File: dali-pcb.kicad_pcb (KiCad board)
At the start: 2 copper layers, 180.5 x 113 mm, 62 parts, among them J1 12-22.5V DC, J10 5V DC, J11 5V DC, J12 5V DC, J13 5V DC, J14 5V DC, J15 GND, J2 DALI BUS, J20 LOLIN-S3 (L), J21 LOLIN-S3 (R), J22 ESP32-S3-DEVKITC-1 (L), J23 ESP32-S3-DEVKITC-1 (R), J24 LOLIN-S3-MINI (L), J25 LOLIN-S3-MINI (R), J26 LOLIN-S2-MINI (L), J27 LOLIN-S2-MINI (R), J3 DALI BUS, J30 FTDI-MCU, J31 UART-DALI, J4 DALI BUS, J40 A10-0, J41 A5-0, J42 A5-5, J43 A2-0, J44 A2-2, J45 A2-4, J46 A2-6, J47 A2-8, J50 D8-11, J51 D4-11, J52 D4-16, J53 D2-11, J54 D2-13, J55 D2-16, J56 D2-18, J60 D1-11, J61 D1-12, J62 D1-13, J63 D1-14, Q1 PZT2222A, Q2 MMBT2222A, U1 TCLT1000, U2 TCLT1000

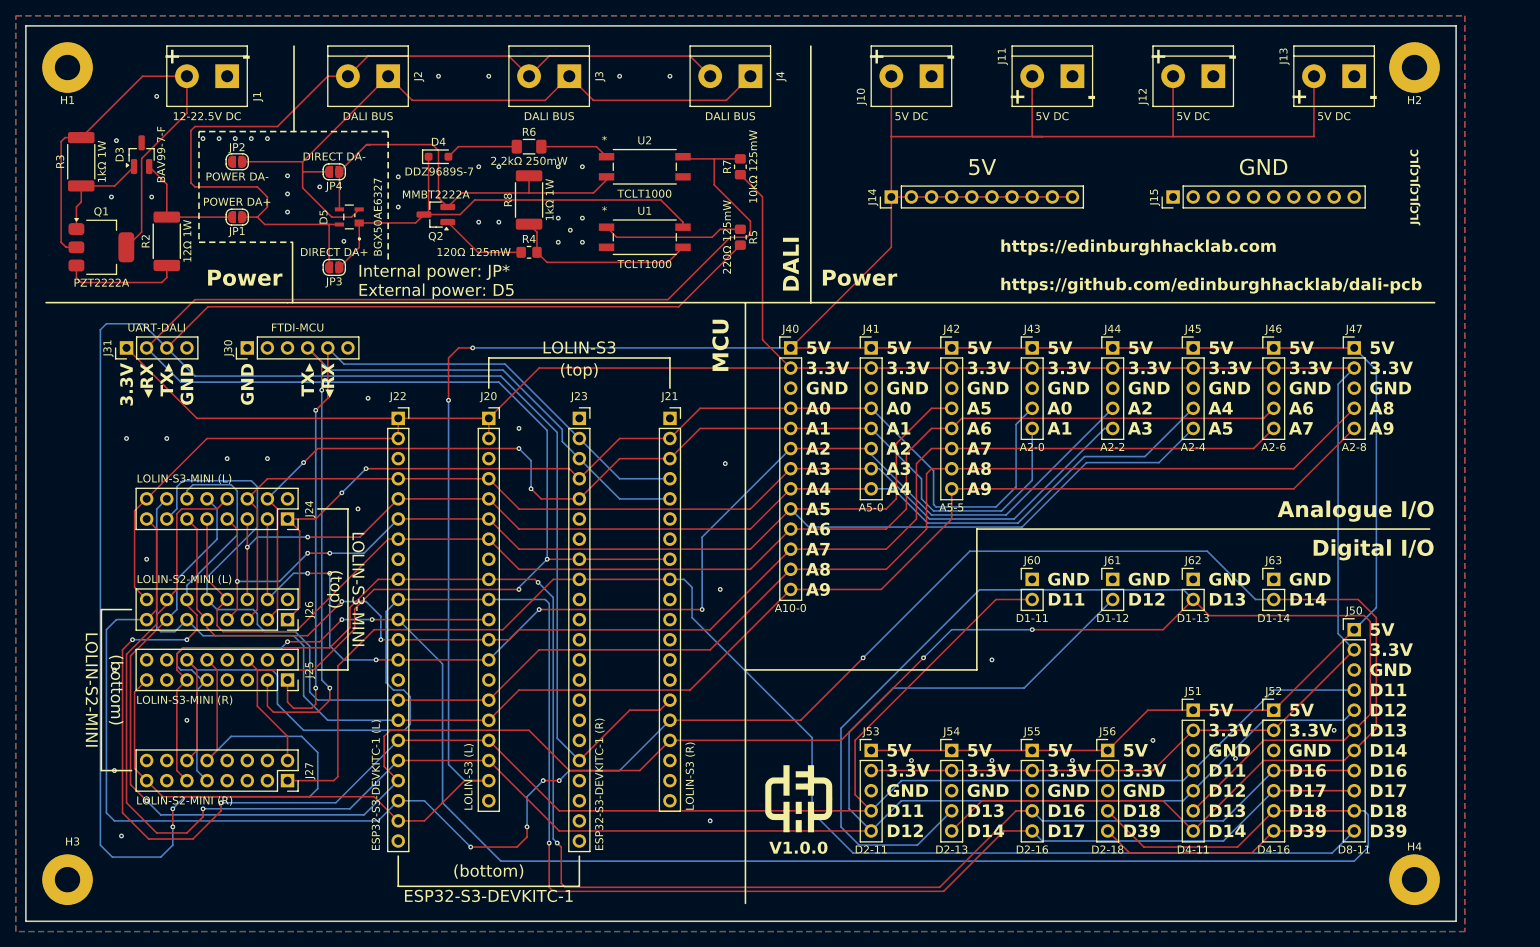
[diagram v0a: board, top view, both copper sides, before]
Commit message: Remove the kitchen sink
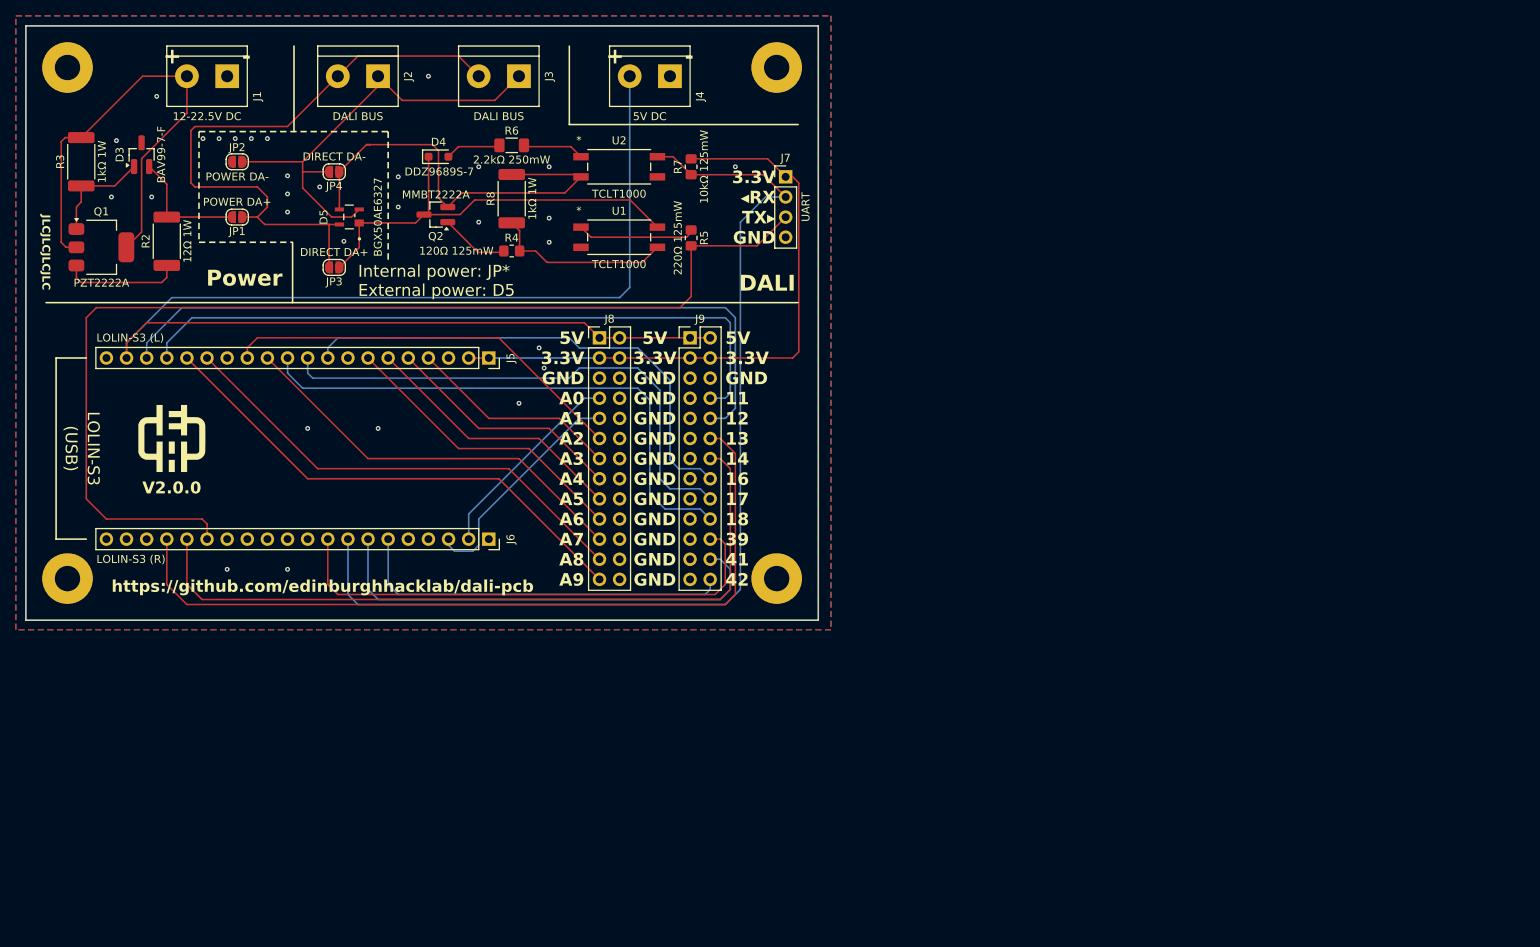
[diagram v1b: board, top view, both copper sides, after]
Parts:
- removed J11, J12, J13: 5V DC, TerminalBlock:TerminalBlock_bornier-2_P5.08mm
- removed J14: 5V DC, Connector_PinHeader_2.54mm:PinHeader_1x10_P2.54mm_Vertical
- removed J15: GND, Connector_PinHeader_2.54mm:PinHeader_1x10_P2.54mm_Vertical
- removed J22: ESP32-S3-DEVKITC-1 (L), Connector_PinSocket_2.54mm:PinSocket_1x22_P2.54mm_Vertical
- removed J23: ESP32-S3-DEVKITC-1 (R), Connector_PinSocket_2.54mm:PinSocket_1x22_P2.54mm_Vertical
- removed J24: LOLIN-S3-MINI (L), Connector_PinSocket_2.54mm:PinSocket_2x08_P2.54mm_Vertical
- removed J25: LOLIN-S3-MINI (R), Connector_PinSocket_2.54mm:PinSocket_2x08_P2.54mm_Vertical
- removed J26: LOLIN-S2-MINI (L), Connector_PinSocket_2.54mm:PinSocket_2x08_P2.54mm_Vertical
- removed J27: LOLIN-S2-MINI (R), Connector_PinSocket_2.54mm:PinSocket_2x08_P2.54mm_Vertical
- removed J30: FTDI-MCU, Connector_PinHeader_2.54mm:PinHeader_1x06_P2.54mm_Vertical
- removed the J4 at (106.7, 21.6)
- removed J41: A5-0, Connector_PinHeader_2.54mm:PinHeader_1x08_P2.54mm_Vertical
- removed J42: A5-5, Connector_PinHeader_2.54mm:PinHeader_1x08_P2.54mm_Vertical
- removed J43: A2-0, Connector_PinHeader_2.54mm:PinHeader_1x05_P2.54mm_Vertical
- removed J44: A2-2, Connector_PinHeader_2.54mm:PinHeader_1x05_P2.54mm_Vertical
- removed J45: A2-4, Connector_PinHeader_2.54mm:PinHeader_1x05_P2.54mm_Vertical
- removed J46: A2-6, Connector_PinHeader_2.54mm:PinHeader_1x05_P2.54mm_Vertical
- removed J47: A2-8, Connector_PinHeader_2.54mm:PinHeader_1x05_P2.54mm_Vertical
- removed J51: D4-11, Connector_PinHeader_2.54mm:PinHeader_1x07_P2.54mm_Vertical
- removed J52: D4-16, Connector_PinHeader_2.54mm:PinHeader_1x07_P2.54mm_Vertical
- removed J53: D2-11, Connector_PinHeader_2.54mm:PinHeader_1x05_P2.54mm_Vertical
- removed J54: D2-13, Connector_PinHeader_2.54mm:PinHeader_1x05_P2.54mm_Vertical
- removed J55: D2-16, Connector_PinHeader_2.54mm:PinHeader_1x05_P2.54mm_Vertical
- removed J56: D2-18, Connector_PinHeader_2.54mm:PinHeader_1x05_P2.54mm_Vertical
- removed J60: D1-11, Connector_PinHeader_2.54mm:PinHeader_1x02_P2.54mm_Vertical
- removed J61: D1-12, Connector_PinHeader_2.54mm:PinHeader_1x02_P2.54mm_Vertical
- removed J62: D1-13, Connector_PinHeader_2.54mm:PinHeader_1x02_P2.54mm_Vertical
- removed J63: D1-14, Connector_PinHeader_2.54mm:PinHeader_1x02_P2.54mm_Vertical
- J7: renamed from J31; value UART-DALI -> UART
- J8: renamed from J40; footprint Connector_PinHeader_2.54mm:PinHeader_1x13_P2.54mm_Vertical -> Connector_PinHeader_2.54mm:PinHeader_2x13_P2.54mm_Vertical
- J9: renamed from J50; footprint Connector_PinHeader_2.54mm:PinHeader_1x11_P2.54mm_Vertical -> Connector_PinHeader_2.54mm:PinHeader_2x13_P2.54mm_Vertical
- moved J9 91.6 mm to (99.1, 54.6)
- moved EHLAB 91.3 mm to (33.7, 67.3)
- moved H4 89.0 mm to (110.0, 85.0)
- moved J7 85.9 mm to (111.1, 34.3), turned to 0 degrees
- moved H2 80.5 mm to (110.0, 20.5)
- moved H3 38.0 mm to (20.5, 85.0), turned to -90 degrees
- moved J4 33.0 mm to (96.5, 21.6)
- moved J6 27.5 mm to (73.7, 80.0), turned to -90 degrees
- moved J8 24.2 mm to (87.6, 54.6)
- moved J5 7.62 mm to (73.7, 57.1), turned to -90 degrees
- moved J3 6.36 mm to (77.5, 21.6)
- moved R5 6.22 mm to (99.2, 42.0)
- moved R7 6.21 mm to (99.2, 33.0), turned to -90 degrees
- moved U1 3.23 mm to (90.1, 41.9)
- moved U2 3.23 mm to (90.1, 33.0)
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- renumbered J10 to J4, J20 to J5, J21 to J6
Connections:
- J6 pad 4: /IO/FTDI_MCU_RXD -> unconnected-(J6-Pin_4-Pad4)
- J6 pad 5: /IO/FTDI_MCU_TXD -> unconnected-(J6-Pin_5-Pad5)
- J6 pad 6: unconnected-(J21-Pin_6-Pad6) -> /IO/IO_D42
- J6 pad 7: unconnected-(J21-Pin_7-Pad7) -> /IO/IO_D41
- J8 pad 10: /IO/IO_A6 -> GND
- J8 pad 11: /IO/IO_A7 -> /IO/IO_A2
- J8 pad 12: /IO/IO_A8 -> GND
- J8 pad 13: /IO/IO_A9 -> /IO/IO_A3
- J8 pad 2: +3.3V -> +5V
- J8 pad 3: GND -> +3.3V
- J8 pad 4: /IO/IO_A0 -> +3.3V
- J8 pad 5: /IO/IO_A1 -> GND
- J8 pad 6: /IO/IO_A2 -> GND
- J8 pad 7: /IO/IO_A3 -> /IO/IO_A0
- J8 pad 8: /IO/IO_A4 -> GND
- J8 pad 9: /IO/IO_A5 -> /IO/IO_A1
- J9 pad 10: /IO/IO_D18 -> /IO/IO_D12
- J9 pad 11: /IO/IO_D39 -> GND
- J9 pad 2: +3.3V -> +5V
- J9 pad 3: GND -> +3.3V
- J9 pad 4: /IO/IO_D11 -> +3.3V
- J9 pad 5: /IO/IO_D12 -> GND
- J9 pad 6: /IO/IO_D13 -> GND
- J9 pad 7: /IO/IO_D14 -> GND
- J9 pad 8: /IO/IO_D16 -> /IO/IO_D11
- J9 pad 9: /IO/IO_D17 -> GND
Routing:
- net +5V: track 478.4 -> 172.4 mm, vias 2 -> 0
- net +3.3V: track 346.7 -> 78.1 mm
- net /IO/IO_D13: track 342.0 -> 100.8 mm, vias 3 -> 0
- net /IO/IO_D14: track 304.6 -> 93.9 mm, vias 5 -> 0
- net /DALI/DALI_TX: track 332.3 -> 138.6 mm, vias 2 -> 0
- net /IO/IO_D11: track 271.0 -> 86.3 mm, vias 3 -> 0
- net /IO/IO_D18: track 247.3 -> 69.8 mm, vias 3 -> 0
- net /IO/IO_D12: track 270.3 -> 93.7 mm, vias 1 -> 0
- net /IO/IO_D17: track 229.7 -> 66.9 mm, vias 1 -> 0
- net /IO/IO_D16: track 215.3 -> 63.3 mm, vias 2 -> 0
- net /IO/IO_D39: track 210.0 -> 64.2 mm
- net /IO/IO_A8: track 205.8 -> 60.1 mm
- net /IO/IO_A5: track 177.1 -> 34.0 mm, vias 3 -> 0
- net /IO/IO_A9: track 195.2 -> 63.6 mm
- net /IO/IO_A6: track 167.6 -> 37.6 mm
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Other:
- board size 180.5 x 113 mm -> 100 x 75 mm
- board text added: "(USB)"
- board text added: "5V 3.3V GND 11 12 13 14 16 17 18 39 41 42"
- board text added: "5V 3.3V GND GND GND GND GND GND GND GND GND GND GND"
- board text added: "V2.0.0"
- board text added: "https://github.com/edinburghhacklab/dali-pcb"
- board text removed: "(bottom)"
- board text removed: "(top)"
- board text removed: "5V"
- board text removed: "5V 3.3V GND A0 A1"
- board text removed: "5V 3.3V GND A0 A1 A2 A3 A4"
- board text removed: "5V 3.3V GND A2 A3"
- board text removed: "5V 3.3V GND A4 A5"
- board text removed: "5V 3.3V GND A5 A6 A7 A8 A9"
- board text removed: "5V 3.3V GND A6 A7"
- board text removed: "5V 3.3V GND A8 A9"
- board text removed: "5V 3.3V GND D11 D12"
- board text removed: "5V 3.3V GND D11 D12 D13 D14"
- board text removed: "5V 3.3V GND D11 D12 D13 D14 D16 D17 D18 D39"
- board text removed: "5V 3.3V GND D13 D14"
- board text removed: "5V 3.3V GND D16 D17"
- board text removed: "5V 3.3V GND D16 D17 D18 D39"
- board text removed: "5V 3.3V GND D18 D39"
- board text removed: "Analogue I/O"
- board text removed: "Digital I/O"
- board text removed: "ESP32-S3-DEVKITC-1"
- board text removed: "GND"
- board text removed: "GND D11"
- board text removed: "GND D12"
- board text removed: "GND D13"
- board text removed: "GND D14"
- board text removed: "GND TX▸ ◂RX"
- board text removed: "LOLIN-S2-MINI"
- board text removed: "LOLIN-S3-MINI"
- board text removed: "MCU"
- board text removed: "V1.0.0"
- board text removed: "https://edinburghhacklab.com https://github.com/edinburghhacklab/dali-pcb"
